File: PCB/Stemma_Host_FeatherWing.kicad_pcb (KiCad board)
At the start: 2 copper layers, 50.8 x 22.9 mm, 17 parts, among them J1 STEMMA, J2 STEMMA, J3 STEMMA-QT, J4 STEMMA-QT, M1 Feather_M4_Express, U1 BSS138DW-Y-F_ALT, U2 AP2112-3.3

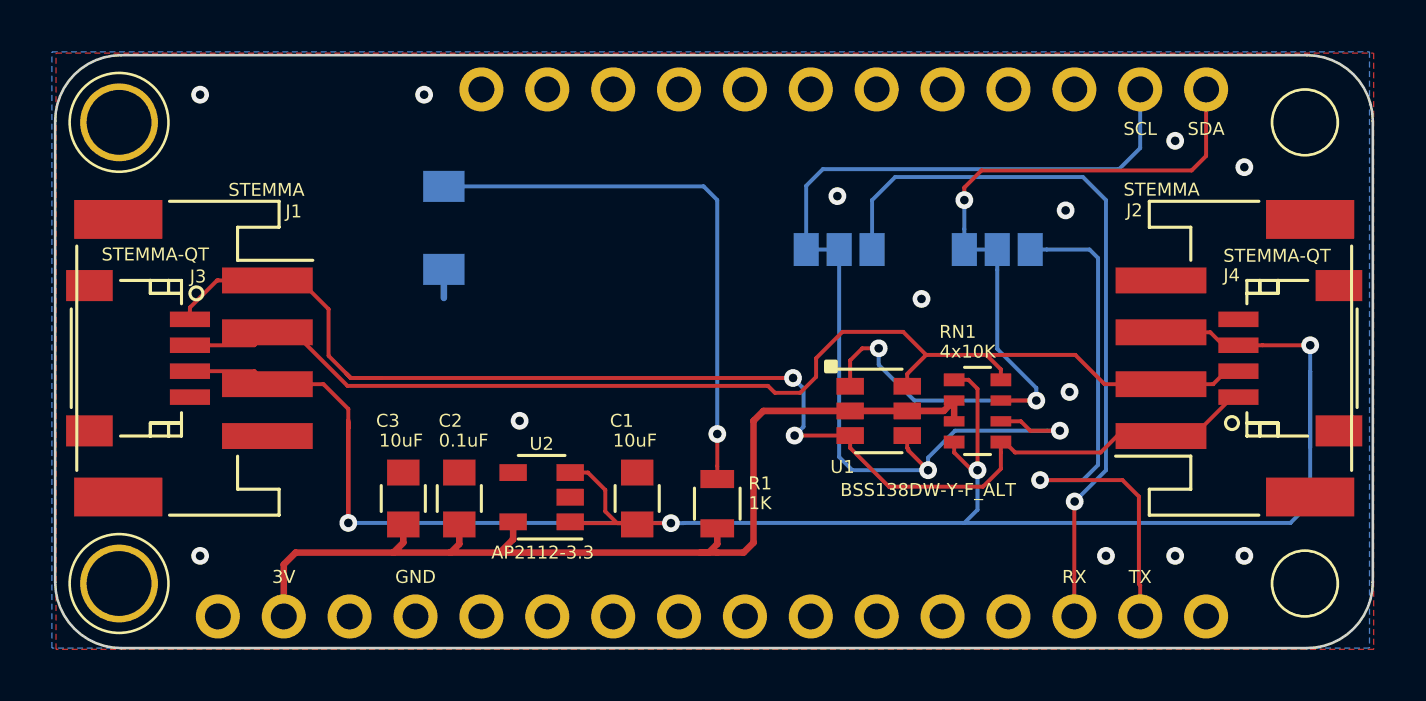
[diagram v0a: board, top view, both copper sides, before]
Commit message: update with initial design
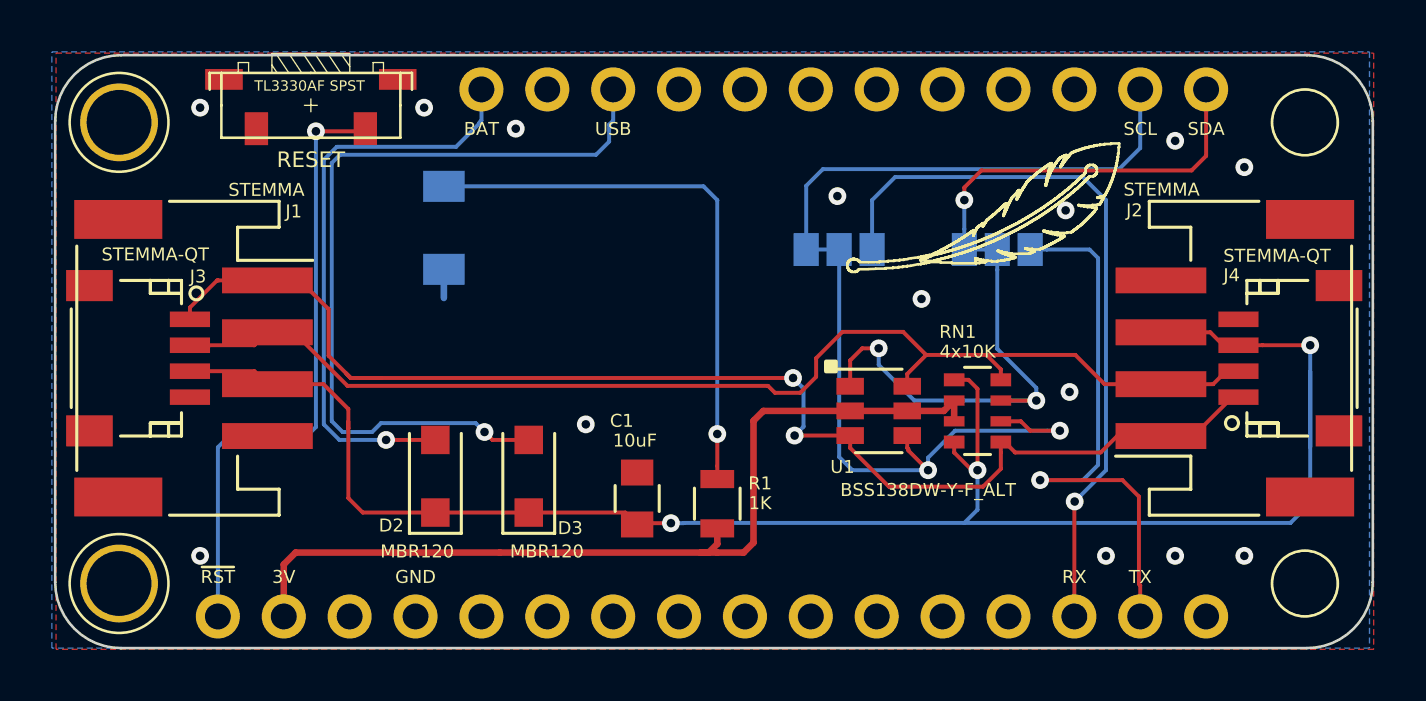
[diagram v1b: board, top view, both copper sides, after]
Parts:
- removed C2: 0.1uF, Capacitors_SMD:C_0805
- removed C3: 10uF, Capacitors_SMD:C_0805
- removed U2: AP2112-3.3, TO_SOT_Packages_SMD:SOT-23-5
- added D2: MBR120, Diodes_SMD:D_SOD-123F, F.Cu at (122.1, 99.8)
- added D3: MBR120, Diodes_SMD:D_SOD-123F, F.Cu at (125.7, 99.8)
- added SW1: RESET, Adafruit:TL3330AF_SPST_BUTTON_RT-ANGLE_7.8mm_2.5mm_2.5mm, F.Cu at (117.3, 85.5)
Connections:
- M1 pad 1: (no net) -> /~RST
- M1 pad 17: (no net) -> /BAT
- M1 pad 19: (no net) -> /USB
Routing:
- net /USB: track 0.00 -> 31.2 mm, vias 0 -> 1
- net /~RST: track 0.00 -> 24.0 mm, vias 0 -> 1
- net /BAT: track 0.00 -> 22.7 mm, vias 0 -> 1
- net /+V: track 84.3 -> 72.1 mm, vias 4 -> 3
- net +3V3: track 39.4 -> 35.4 mm
- net GND: vias 13 -> 14
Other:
- board text added: "2019-11-26 v01"
- board text added: "A Feather-powered Stemma FeatherWing. The host Feather provides 3.3V or ~5V for the Stemma connector."
- board text added: "Stemma Host FeatherWing"
- board text removed: "2019-11-26 v02"
- board text removed: "A Stemma-powered interface backpack for FeatherWings. The Stemma connector provides +3.3V to the attached Wing."
- board text removed: "StemmaWing Backpack"
